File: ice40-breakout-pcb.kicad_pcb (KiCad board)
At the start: 2 copper layers, 56 x 78.3 mm, 59 parts, among them J1 USB_B_Micro, J2 USB_Break_Out, J3 Conn_02x16_Odd_Even, J4 Conn_02x16_Odd_Even, J5 Conn_02x16_Odd_Even, J6 Conn_02x04_Odd_Even, U1 SIT2001BI-S2-33E-12.000000G, U2 TLV73333PDBV, U3 TLV73312PDBV, U4 AT25SF081-SHD-X, U5 ICE40HX4K-TQ144

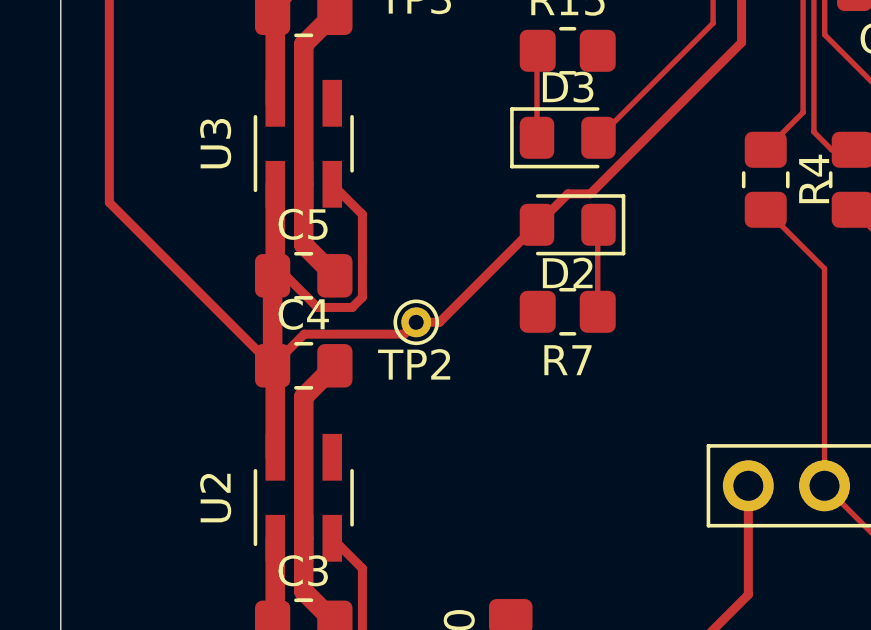
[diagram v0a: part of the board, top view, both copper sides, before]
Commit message: Cosmetic tweak.
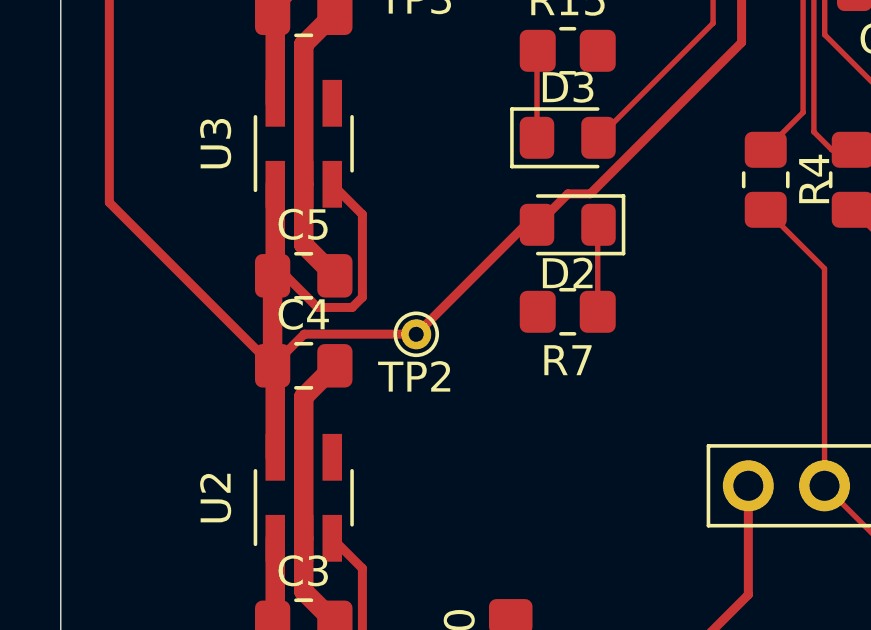
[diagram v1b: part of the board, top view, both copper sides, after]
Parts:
- moved TP2 0.40 mm to (103.8, 118.7)
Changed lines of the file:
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@@
     (add_net VPP_2V5)
+  )
+  (module TestPoint:TestPoint_THTPad_D1.0mm_Drill0.5mm (layer F.Cu)
+    (at 103.85 118.65 180)
+    (descr "THT pad as test Point, diameter 1.0mm, hole diameter 0.5mm")
+    (tags "test point THT pad")
+    (attr virtual)
+    (fp_text reference TP2 (at 0 -1.448) (layer F.SilkS)
+      (effects (font (size 1 1) (thickness 0.15)))
+    )
+    (fp_text value TestPoint (at 0 1.55) (layer F.Fab)
+      (effects (font (size 1 1) (thickness 0.15)))
+    )
+    (fp_circle (center 0 0) (end 1 0) (layer F.CrtYd) (width 0.05))
+    (fp_circle (center 0 0) (end 0 0.7) (layer F.SilkS) (width 0.12))
+    (fp_text user %R (at 0 -1.45) (layer F.Fab)
+      (effects (font (size 1 1) (thickness 0.15)))
+    )
+    (pad 1 thru_hole circle (at 0 0 180) (size 1 1) (drill 0.5) (layers *.Cu *.Mask)
+      (net 3 +3V3))
   )
   (module Connector_PinHeader_2.54mm:PinHeader_2x04_P2.54mm_Vertical (layer F.Cu)
@@
     (pad 1 thru_hole circle (at 0 0 180) (size 1 1) (drill 0.5) (layers *.Cu *.Mask)
       (net 4 +1V2))
-  )
-  (module TestPoint:TestPoint_THTPad_D1.0mm_Drill0.5mm (layer F.Cu)
-    (at 103.85 118.25 180)
-    (descr "THT pad as test Point, diameter 1.0mm, hole diameter 0.5mm")
-    (tags "test point THT pad")
-    (attr virtual)
-    (fp_text reference TP2 (at 0 -1.448) (layer F.SilkS)
-      (effects (font (size 1 1) (thickness 0.15)))
-    )
-    (fp_text value TestPoint (at 0 1.55) (layer F.Fab)
-      (effects (font (size 1 1) (thickness 0.15)))
-    )
-    (fp_circle (center 0 0) (end 1 0) (layer F.CrtYd) (width 0.05))
-    (fp_circle (center 0 0) (end 0 0.7) (layer F.SilkS) (width 0.12))
-    (fp_text user %R (at 0 -1.45) (layer F.Fab)
-      (effects (font (size 1 1) (thickness 0.15)))
-    )
-    (pad 1 thru_hole circle (at 0 0 180) (size 1 1) (drill 0.5) (layers *.Cu *.Mask)
-      (net 3 +3V3))
   )
   (module TestPoint:TestPoint_THTPad_D1.0mm_Drill0.5mm (layer F.Cu)
@@
   (segment (start 100.55975 117.75501) (end 101.71525 117.75501) (width 0.3) (layer F.Cu) (net 3))
   (segment (start 99.0625 116.7) (end 99.50474 116.7) (width 0.3) (layer F.Cu) (net 3))
-  (segment (start 103.45501 118.64499) (end 103.85 118.25) (width 0.3) (layer F.Cu) (net 3))
-  (segment (start 100.11751 118.64499) (end 103.45501 118.64499) (width 0.3) (layer F.Cu) (net 3))
-  (segment (start 99.0625 119.7) (end 100.11751 118.64499) (width 0.3) (layer F.Cu) (net 3))
-  (segment (start 104.625 118.25) (end 107.875 115) (width 0.3) (layer F.Cu) (net 3))
-  (segment (start 103.85 118.25) (end 104.625 118.25) (width 0.3) (layer F.Cu) (net 3))
   (segment (start 120.13498 99.23498) (end 118.9 98) (width 0.3) (layer F.Cu) (net 3))
   (segment (start 116.45 98) (end 115.75 98.7) (width 0.3) (layer F.Cu) (net 3))
@@
   (segment (start 140.70501 109.19499) (end 142.999012 109.19499) (width 0.3) (layer F.Cu) (net 3))
   (segment (start 139.75 110.15) (end 140.70501 109.19499) (width 0.3) (layer F.Cu) (net 3))
+  (segment (start 107.5 115) (end 103.85 118.65) (width 0.3) (layer F.Cu) (net 3))
+  (segment (start 107.875 115) (end 107.5 115) (width 0.3) (layer F.Cu) (net 3))
+  (segment (start 100.11751 118.64499) (end 103.84499 118.64499) (width 0.3) (layer F.Cu) (net 3))
+  (segment (start 103.84499 118.64499) (end 103.85 118.65) (width 0.3) (layer F.Cu) (net 3))
+  (segment (start 99.0625 119.7) (end 100.11751 118.64499) (width 0.3) (layer F.Cu) (net 3))
   (via (at 114.9 94.25) (size 0.8) (drill 0.4) (layers F.Cu B.Cu) (net 4))
   (via (at 116.6 94.25) (size 0.8) (drill 0.4) (layers F.Cu B.Cu) (net 4))
